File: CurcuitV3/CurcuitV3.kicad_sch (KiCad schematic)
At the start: 96 parts, among them IC1 AS5600-ASOT, J1 Conn_01x07, J2 Conn_01x03, J3 Conn_01x02, J4 Conn_01x02, Q1 Q_NMOS_DGS, Q2 Q_NMOS_DGS, Q3 Q_NMOS_DGS, Q4 Q_NMOS_DGS, Q5 Q_NMOS_DGS, Q6 Q_NMOS_DGS, SW1 SW_Push, SW2 SW_Push, U1 DRV8300DPWR, U2 STM32F303K8Tx, U3 MCP9700x-ETT, U4 LM66100DCK, U5 INA180A2, U6 INA180A2, U7 AP7375-3.3, Y2 CSTNE16M0V530000R0

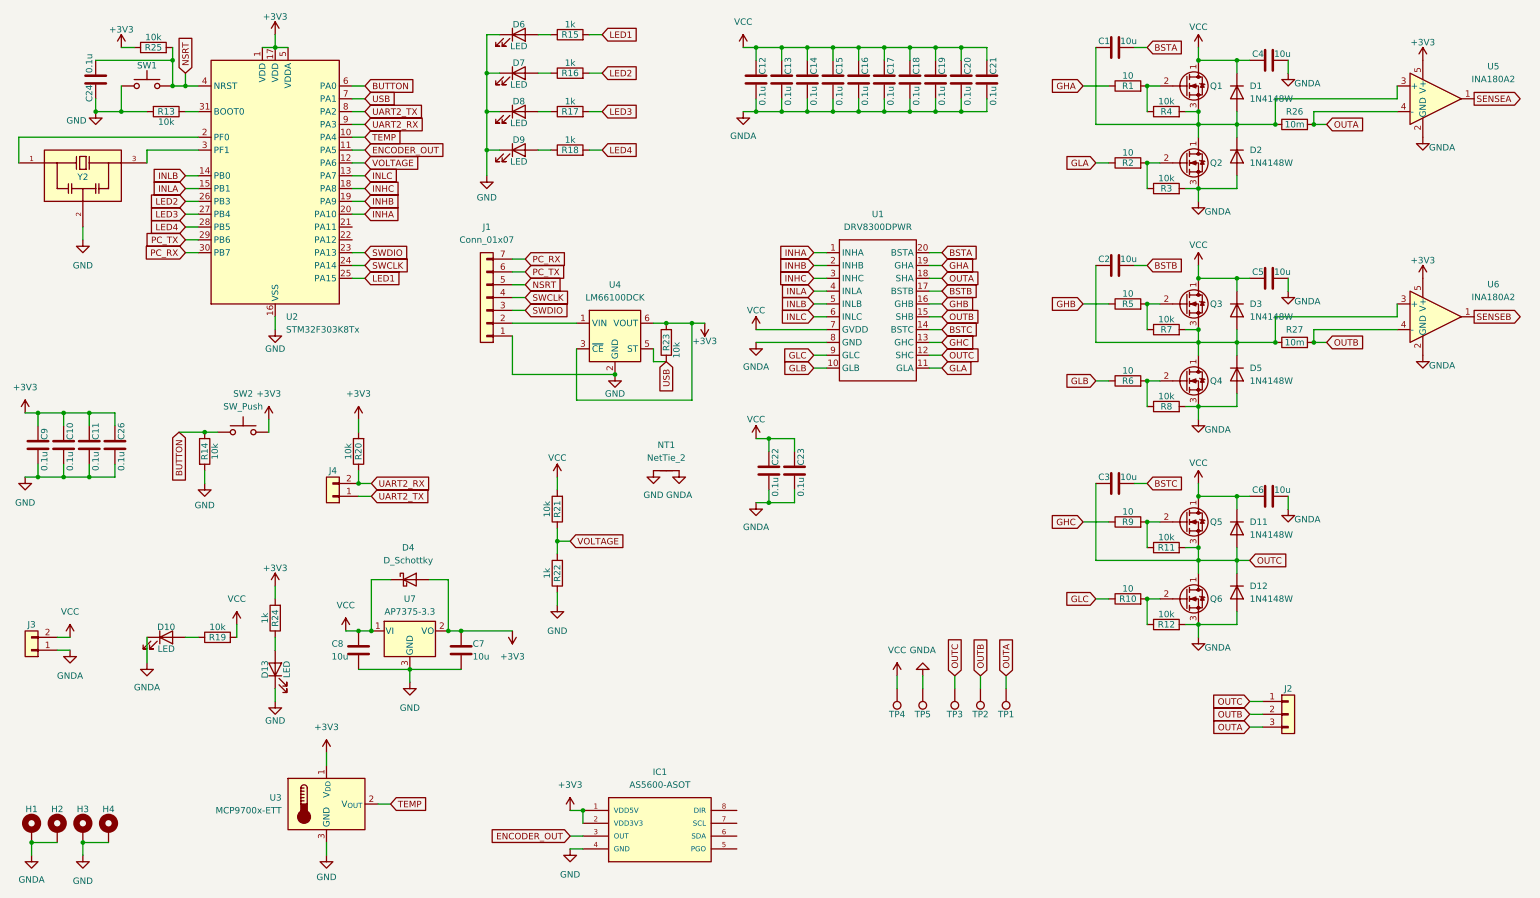
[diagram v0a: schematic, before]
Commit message: 回路ほぼ完成
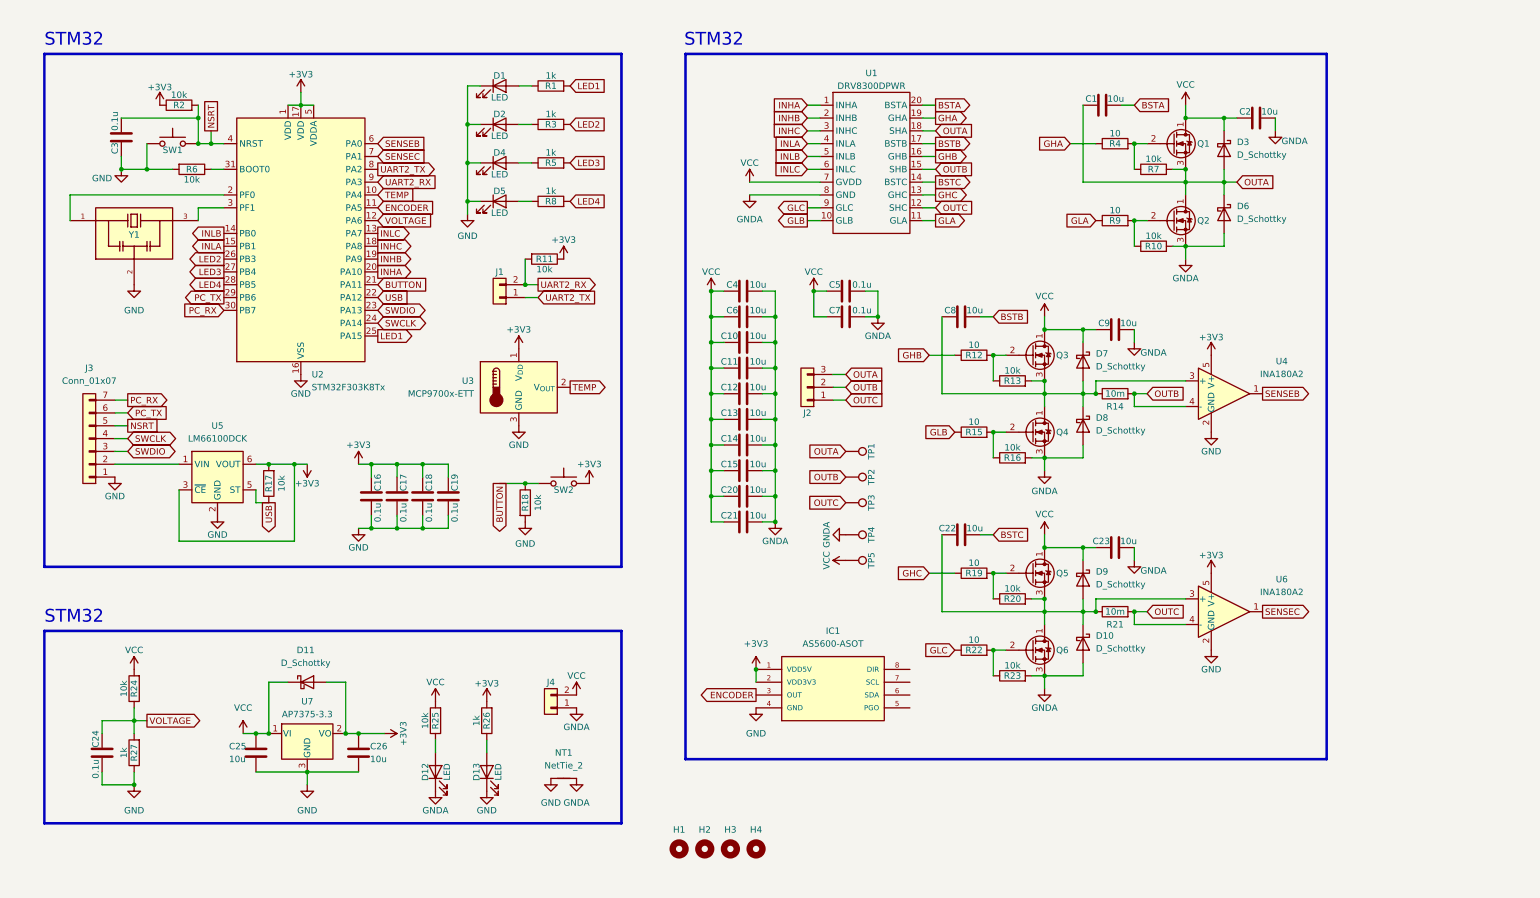
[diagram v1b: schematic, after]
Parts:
- removed D1, D11, D12, D2, D3, D5: 1N4148W, Diode_SMD:D_SOD-123, symbol Diode:1N4148W
- removed H1, H2, H3, H4: MountingHole_Pad, MountingHole:MountingHole_3.2mm_M3_ISO14580_Pad_TopBottom, symbol Mechanical:MountingHole_Pad
- removed U5: INA180A2, Package_TO_SOT_SMD:SOT-23-5, symbol Amplifier_Current:INA180A2
- added C24: 0.1u, Capacitor_SMD:C_0603_1608Metric, symbol Device:C
- added D10, D3, D6, D7, D8, D9: D_Schottky, Diode_SMD:D_SOD-323_HandSoldering, symbol Device:D_Schottky
- added H1, H2, H3, H4: MountingHole, MountingHole:MountingHole_3.2mm_M3_ISO14580_Pad_TopBottom, symbol Mechanical:MountingHole
- added U6: INA180A2, Package_TO_SOT_SMD:SOT-23-5, symbol Amplifier_Current:INA180A2
- C10: renamed from C19; value 0.1u -> 10u
- C11: renamed from C18; value 0.1u -> 10u
- C12: renamed from C17; value 0.1u -> 10u
- C13: renamed from C16; value 0.1u -> 10u
- C14: renamed from C15; value 0.1u -> 10u
- C15: renamed from C14; value 0.1u -> 10u
- C20: renamed from C13; value 0.1u -> 10u
- C21: renamed from C12; value 0.1u -> 10u
- C4: renamed from C21; value 0.1u -> 10u
- C6: renamed from C20; value 0.1u -> 10u
- NT1: footprint NetTie:NetTie-2_SMD_Pad2.0mm -> NetTie:NetTie-2_SMD_Pad0.5mm
- renumbered C9 to C16, C10 to C17, C11 to C18, C26 to C19, C4 to C2, C3 to C22, C6 to C23, C8 to C25, C7 to C26, C24 to C3, C23 to C5, C22 to C7, C2 to C8, C5 to C9, D6 to D1, D4 to D11, D10 to D12, D7 to D2, D8 to D4, D9 to D5, J4 to J1, J1 to J3, J3 to J4, R15 to R1, R3 to R10, R20 to R11, R5 to R12, R7 to R13, R27 to R14, R6 to R15, R8 to R16, R23 to R17, R14 to R18, R9 to R19, R25 to R2, R11 to R20, R26 to R21, R10 to R22, R12 to R23, R21 to R24, R19 to R25, R24 to R26, R22 to R27, R16 to R3, R1 to R4, R17 to R5, R13 to R6, R4 to R7, R18 to R8, R2 to R9, TP5 to TP4, TP4 to TP5, U6 to U4, U4 to U5, Y2 to Y1
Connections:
- net +3V3: now also R11.1, U6.5 (V+); no longer R11.2
- net BUTTON: now also U2.21 (PA11); no longer U2.6 (PA0)
- net GND: now also U4.2 (GND), C24.1, U6.2 (GND)
- net GNDA: now also D10.2 (A), D6.2 (A), D8.2 (A); no longer U4.2 (GND)
- net OUTA: now also C1.1, Q1.3 (S), Q2.1 (D), R7.2, D3.2 (A), D6.1 (K); no longer R21.2
- net OUTC: now also R21.2, U6.4 (-); no longer C22.1, Q5.3 (S), Q6.1 (D), R20.2
- net SENSEB: now also U2.6 (PA0)
- net UART2_RX: now also R11.2; no longer R11.1
- net USB: now also U2.22 (PA12); no longer U2.7 (PA1)
- net VCC: now also D3.1 (K), D7.1 (K), D9.1 (K)
- net VOLTAGE: now also C24.2
- net at C8.1, Q3.3 (S), Q4.1 (D)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: now also D7.2 (A), D8.1 (K)
- net ENCODER_OUT renamed ENCODER
- new net: C22.1, D10.1 (K), D9.2 (A), Q5.3 (S), Q6.1 (D), R20.2, R21.1, U6.3 (+)
- new net SENSEC: U2.7 (PA1), U6.1
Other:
- note added: "STM32"
- moved on the sheet: C1, C10, C11, C12, C13, C14, C15, C16, C17, C18, C19, C2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
